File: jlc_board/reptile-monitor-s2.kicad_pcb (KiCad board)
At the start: 4 copper layers, 38.1 x 76.2 mm, 49 parts, among them J1 USB_C_Receptacle_USB2.0, J2 AC_IN, J3 Conn_01x08, J7 LOAD0, J8 LOAD1, K1 1462041-7, K2 1462041-7, SW1 RESET, SW2 BOOT, U1 ESP32-S2-WROVER, U2 TPS2112PW, U3 AP2112K-3.3, U4 MDC3105LT1G, U5 MDC3105LT1G, Y1 32.768KHz 12.5p

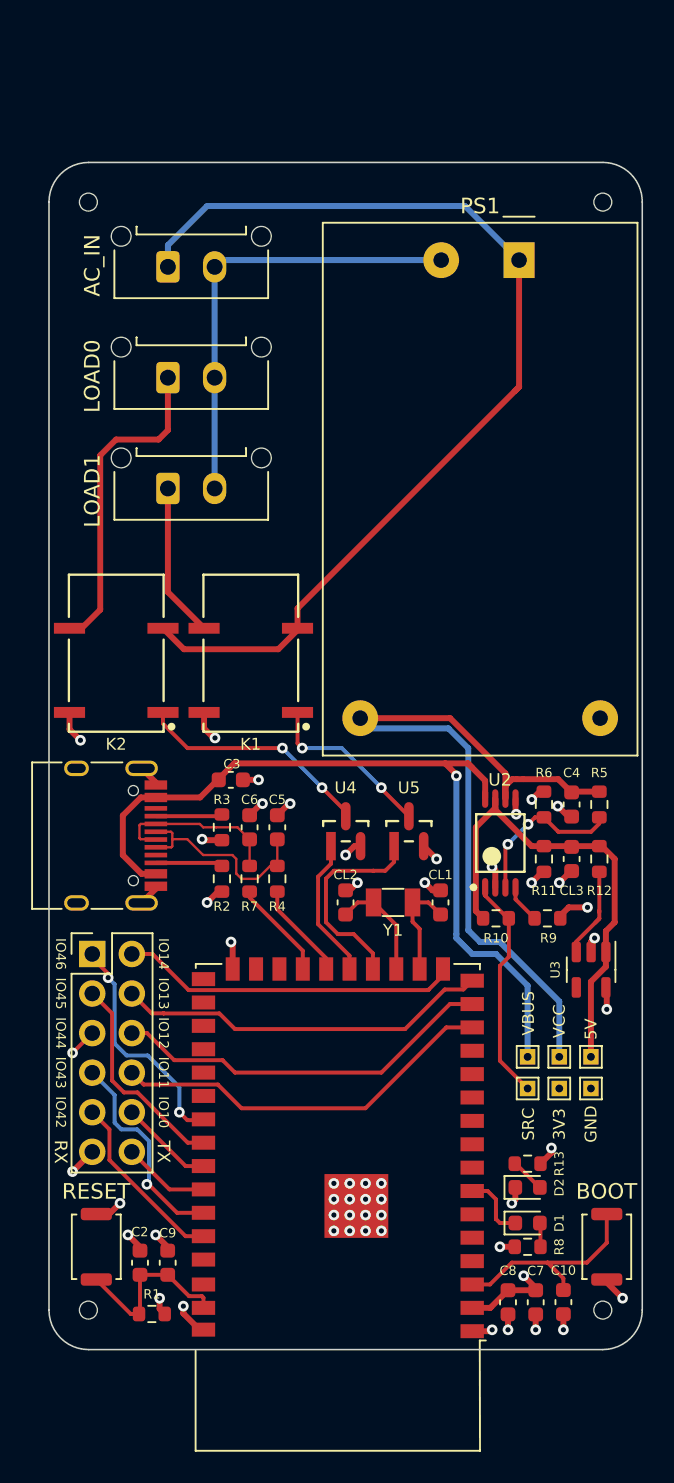
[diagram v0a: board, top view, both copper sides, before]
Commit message: rev2
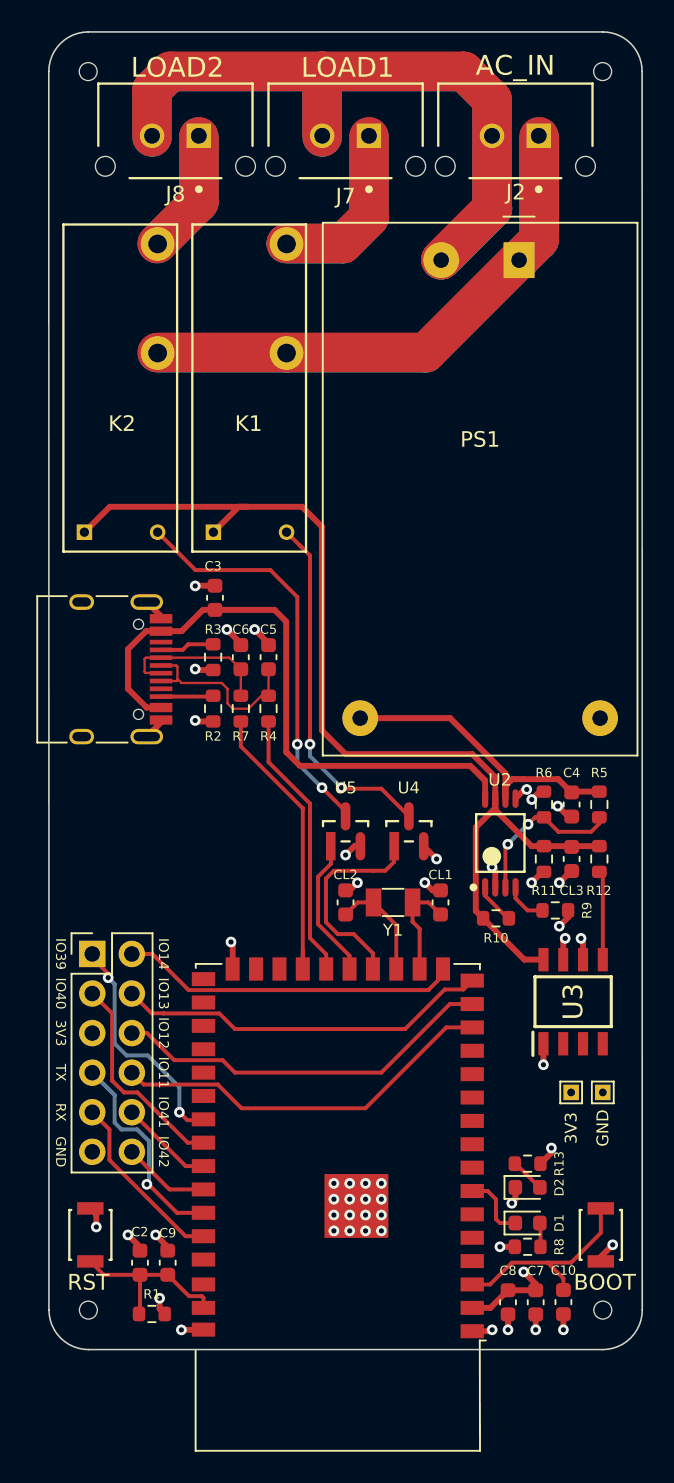
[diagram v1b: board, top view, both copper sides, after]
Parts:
- removed TP2: SRC, TestPoint:TestPoint_THTPad_1.0x1.0mm_Drill0.5mm
- removed TP4: 5V, TestPoint:TestPoint_THTPad_1.0x1.0mm_Drill0.5mm
- removed TP5: VCC, TestPoint:TestPoint_THTPad_1.0x1.0mm_Drill0.5mm
- removed TP6: VBUS, TestPoint:TestPoint_THTPad_1.0x1.0mm_Drill0.5mm
- J2: footprint Connector_Molex:Molex_Micro-Fit_3.0_43650-0215_1x02_P3.00mm_Vertical -> reptile-monitor:Molex-43650-0215-0-0-MFG
- J7: value LOAD0 -> LOAD1; footprint Connector_Molex:Molex_Micro-Fit_3.0_43650-0215_1x02_P3.00mm_Vertical -> reptile-monitor:Molex-43650-0215-0-0-MFG
- J8: value LOAD1 -> LOAD2; footprint Connector_Molex:Molex_Micro-Fit_3.0_43650-0215_1x02_P3.00mm_Vertical -> reptile-monitor:Molex-43650-0215-0-0-MFG
- K1, K2: value 1462041-7 -> ALDP105W; footprint Reptile_Monitor:TE_Connectivity-1462041-7-0-0 -> reptile-monitor:Panasonic-ALDP105W-Manufacturer_Recommended
- R10: value 10K -> 10k
- R9: value 500R -> 500r
- SW1: value RESET -> RST; footprint Reptile_Monitor:Alps_SKRK -> reptile-monitor:Omron-B3U-1000P-MFG
- SW2: footprint Reptile_Monitor:Alps_SKRK -> reptile-monitor:Omron-B3U-1000P-MFG
- U3: footprint Package_TO_SOT_SMD:SOT-23-5 -> SamacSys_Parts:SOIC127P600X170-8N
- moved J2 24.0 mm to (161.3, 41.1)
- moved J8 23.0 mm to (139.4, 41.1)
- moved J7 19.5 mm to (150.4, 41.1)
- moved C3 11.7 mm to (142.0, 71.1), turned to 90 degrees
- moved C5 10.9 mm to (145.4, 74.9)
- moved C6 10.9 mm to (143.6, 74.9)
- moved R2 10.9 mm to (141.9, 78.2)
- moved R3 10.9 mm to (141.9, 74.9)
- moved R4 10.9 mm to (145.4, 78.2)
- moved R7 10.9 mm to (143.6, 78.2)
- moved J1 10.7 mm to (134.5, 75.7)
- moved K1 8.13 mm to (141.9, 66.9)
- moved K2 8.03 mm to (133.6, 66.9)
- moved U5 4.06 mm to (150.4, 86.1)
- moved U4 4.05 mm to (154.4, 86.1)
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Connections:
- J7 pad 1: /LOAD_0 -> /LOAD1
- J8 pad 1: /LOAD_1 -> /LOAD2
- K1 pad 1: Net-(K1-Pad1) -> +5V
- K2 pad 1: Net-(K2-Pad1) -> +5V
- R12 pad 1: +5V -> Net-(R12-Pad1)
- R12 pad 2: Net-(R12-Pad2) -> +5V
- SW1 pad 1: GND -> /EN
- SW1 pad 2: /EN -> GND
- SW2 pad 1: GND -> /IO0
- SW2 pad 2: /IO0 -> GND
- U3 pad 1: +5V -> +3V3
- U3 pad 2: GND -> (no net)
- U3 pad 3: Net-(R12-Pad2) -> (no net)
- U3 pad 5: +3V3 -> Net-(R12-Pad1)
- U4 pad 1: /IO18 -> /IO17
- U4 pad 3: Net-(K2-Pad1) -> Net-(U4-Pad3)
- U5 pad 1: /IO17 -> /IO18
- U5 pad 3: Net-(K1-Pad1) -> Net-(K2-Pad4)
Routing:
- net /AC_N: track 29.6 -> 280.0 mm
- net /AC_L: track 66.1 -> 204.7 mm
- net /LOAD1: track 0.00 -> 67.1 mm
- net /LOAD2: track 0.00 -> 47.7 mm
- net +5V: track 31.5 -> 68.1 mm
- net VCC: track 50.5 -> 19.8 mm
- net Net-(K2-Pad4): track 0.00 -> 26.1 mm, vias 0 -> 2
- net Net-(U4-Pad3): track 0.00 -> 23.2 mm, vias 0 -> 2
- net /LOAD_0: track 20.8 -> 0.00 mm
- net Net-(K2-Pad1): track 15.1 -> 0.00 mm, vias 2 -> 0
- net VBUS: track 53.7 -> 40.9 mm, vias 1 -> 0
- net Net-(R7-Pad2): track 6.38 -> 18.7 mm
- net /PWR_SRC: track 14.5 -> 2.65 mm
- net Net-(R4-Pad2): track 6.27 -> 18.1 mm
- net Net-(K1-Pad1): track 11.1 -> 0.00 mm, vias 2 -> 0
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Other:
- board size 38.1 x 76.2 mm -> 38.1 x 84.6 mm
- board text added: "3V3"
- board text added: "ESP32-S2 Reptile Monitor Mike Pleimann Rev 2 April 2021"
- board text added: "GND"
- board text added: "IO39"
- board text added: "IO40"
- board text added: "IO41"
- board text removed: "ESP32-S2 Reptile Monitor Mike Pleimann v1.0 April 2021"
- board text removed: "IO10"
- board text removed: "IO43"
- board text removed: "IO44"
- board text removed: "IO45"
- board text removed: "IO46"
